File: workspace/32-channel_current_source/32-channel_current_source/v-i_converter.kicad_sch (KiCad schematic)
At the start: 18 parts, among them U2 LMV358, U3 NCV0372

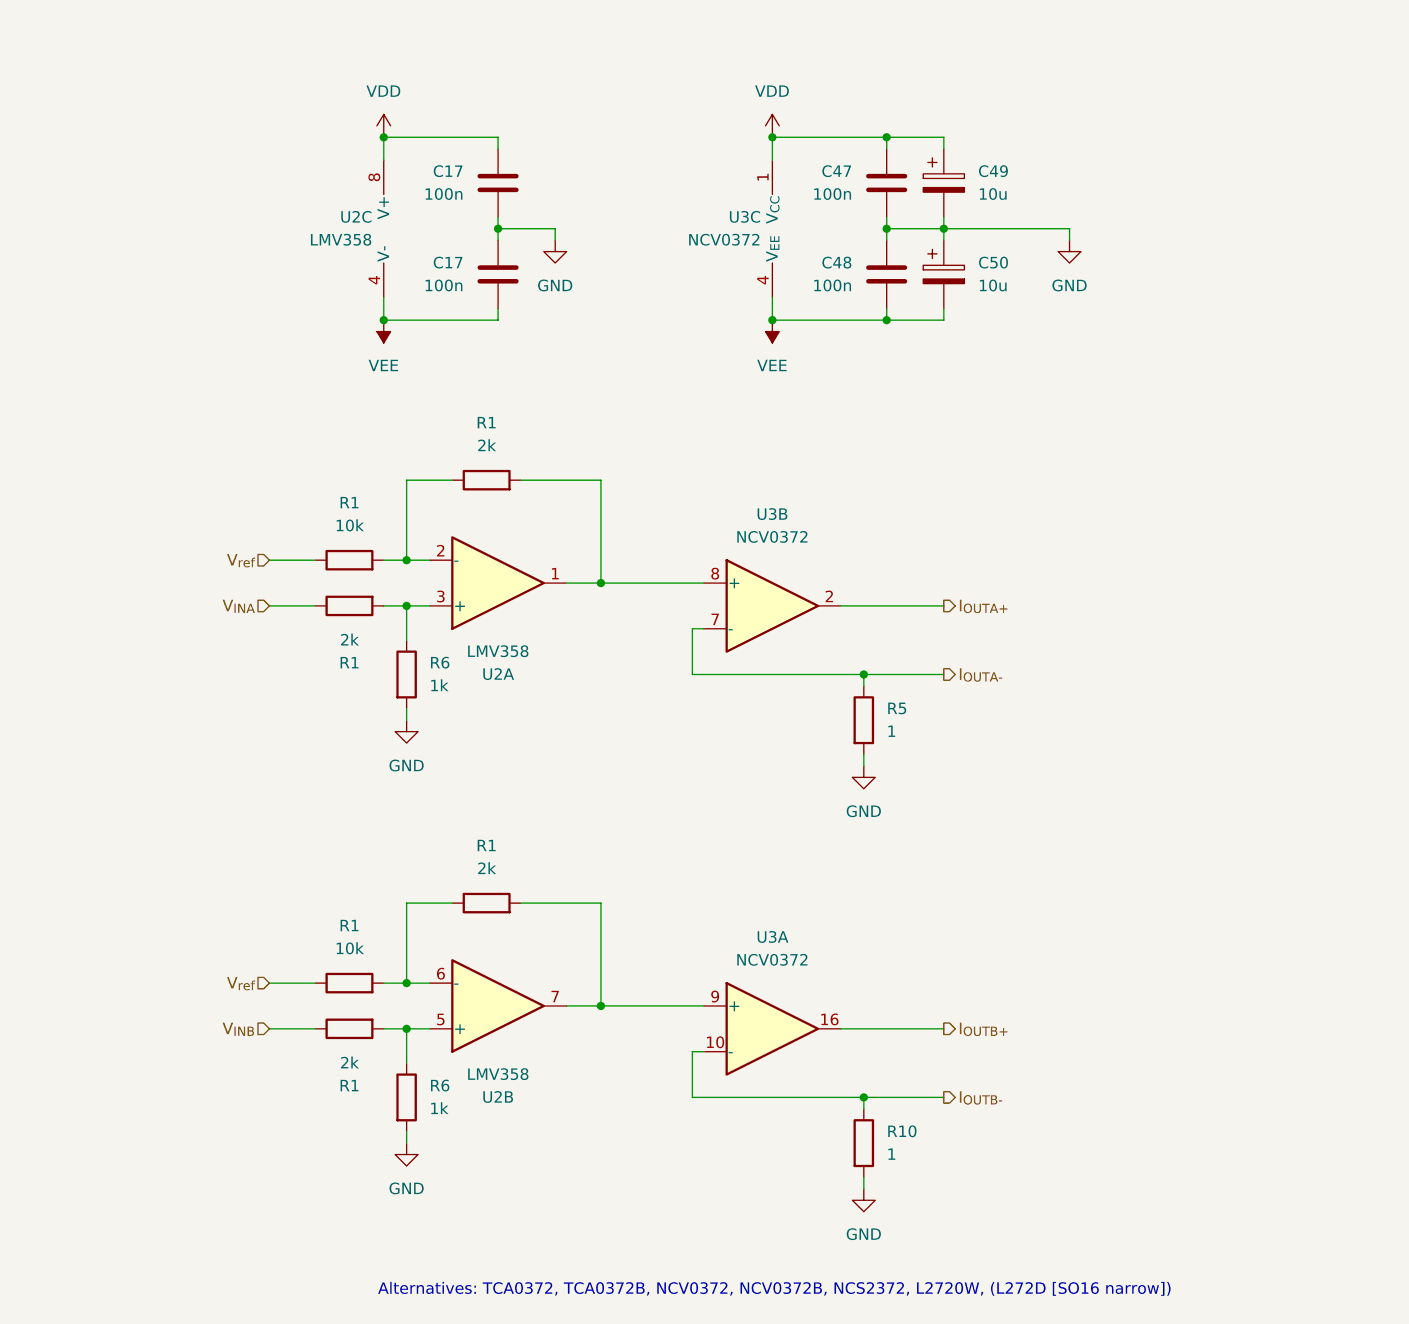
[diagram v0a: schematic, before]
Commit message: Finish Rev 1 of the 32-channel current supply
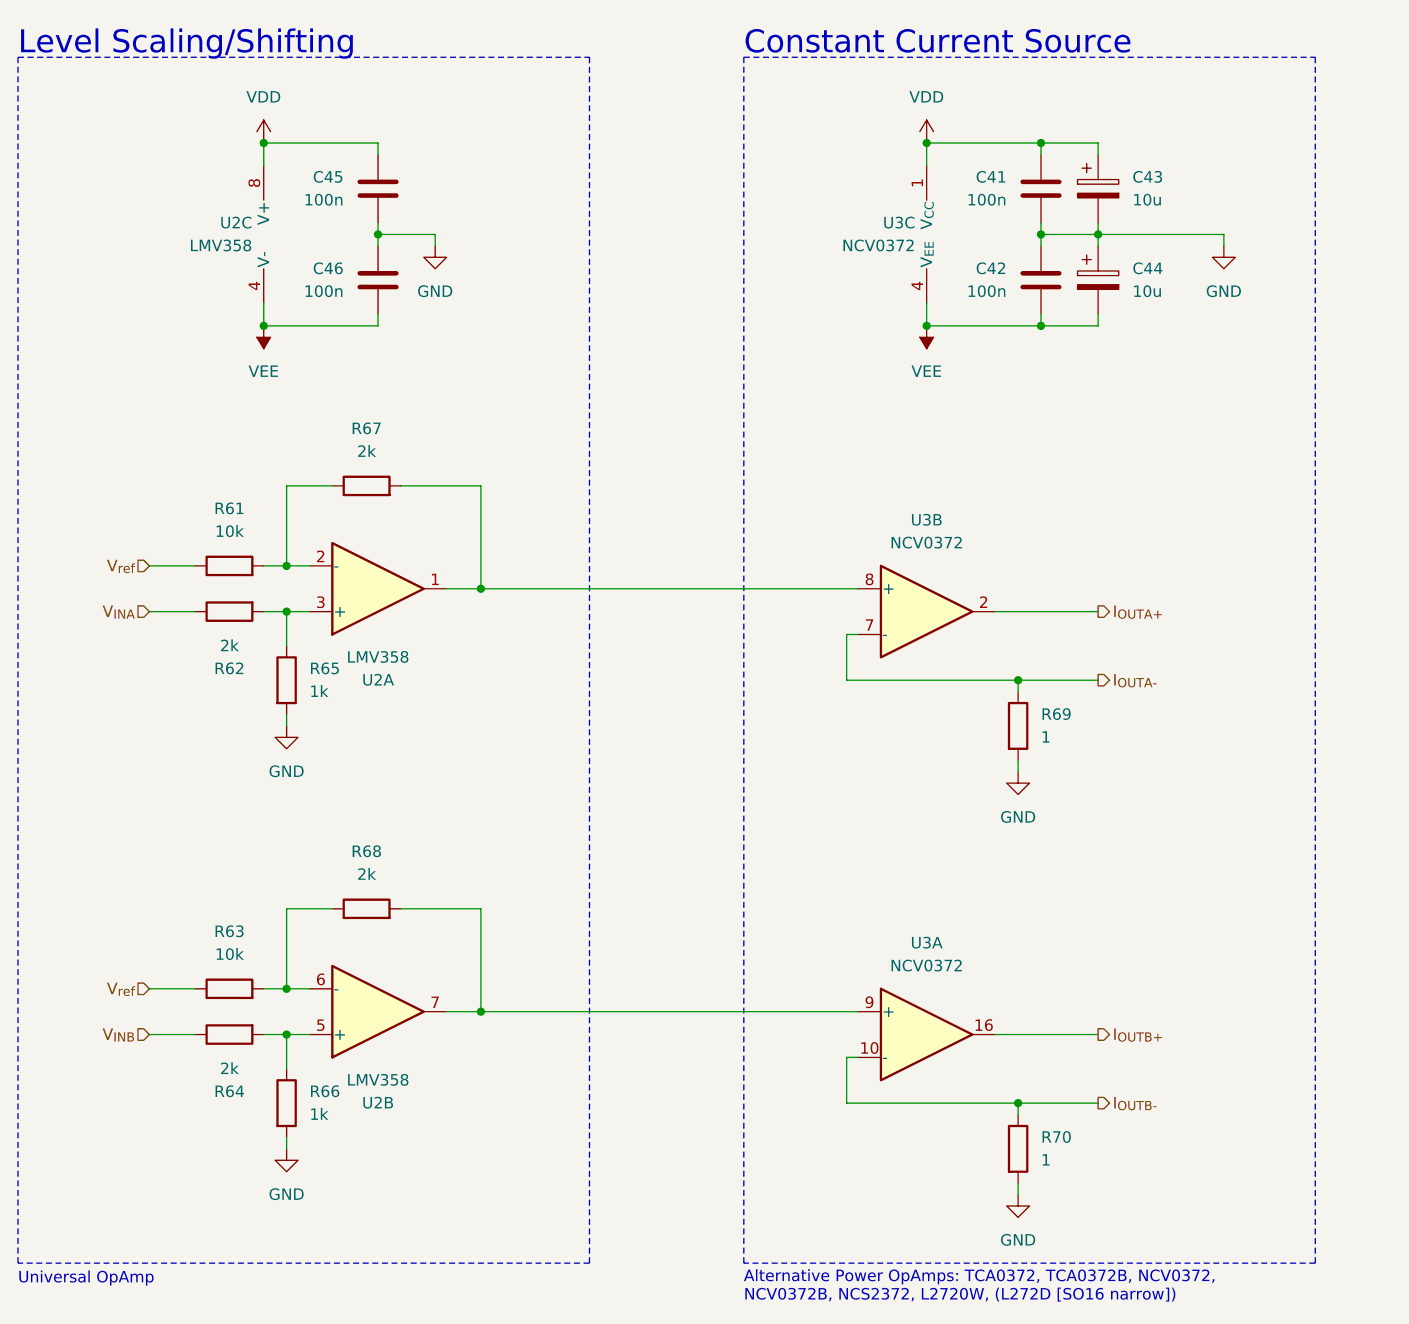
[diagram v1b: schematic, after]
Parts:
- R62, R64, R67, R68: renamed from R1; MPN (none) -> RT0805FRE072KL; Mouser (none) -> 603-RT0805FRE072KL
- R65, R66: renamed from R6; MPN (none) -> RT0805FRE071KL; Mouser (none) -> 603-RT0805FRE071KL
- R69: renamed from R5; Notes (none) -> current sense, precision
- R70: renamed from R10; Notes (none) -> current sense, precision
- U2: MPN (none) -> LMV358IDR; Mouser (none) -> 595-LMV358IDR
- renumbered C47 to C41, C48 to C42, C49 to C43, C50 to C44, C17 to C45, C17 to C46, R1 to R61, R1 to R63
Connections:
- net VEE: no longer U3.12 (V_{EE}), U3.13 (V_{EE}), U3.5 (V_{EE})
- now unconnected: U3.11 (NC), U3.14 (NC), U3.15 (NC), U3.3 (NC), U3.6 (NC)
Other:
- note added: "Alternative Power OpAmps: TCA0372, TCA0372B, NCV0372, NCV0372B, NCS2372, L2720W, (L272D [SO16 narrow])"
- note added: "Constant Current Source"
- note added: "Level Scaling/Shifting"
- note added: "Universal OpAmp"
- note removed: "Alternatives: TCA0372, TCA0372B, NCV0372, NCV0372B, NCS2372, L2720W, (L272D [SO16 narrow])"
- moved on the sheet: C41, C42, C43, C44, C45, C46, R61, R62, R63, R64, R65, R66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
